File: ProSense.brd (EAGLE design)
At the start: 25.5 x 36.7 mm, 24 parts, among them U4 MIC2505 3.3

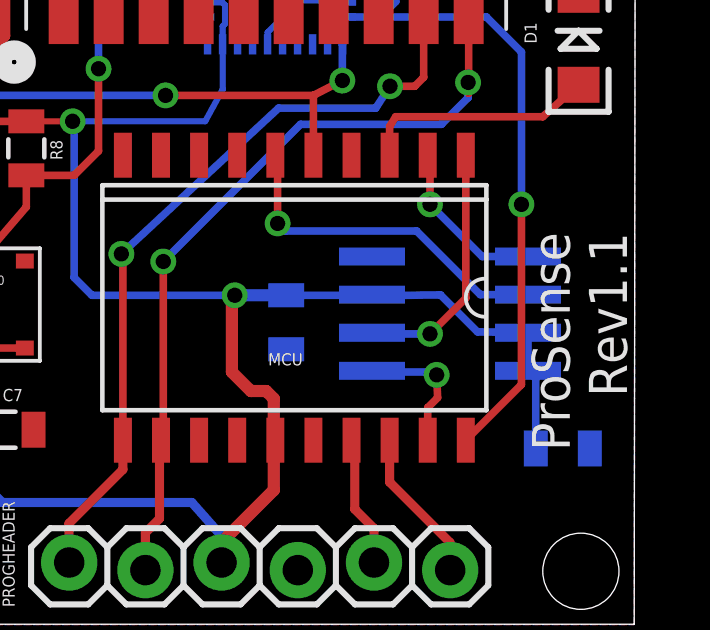
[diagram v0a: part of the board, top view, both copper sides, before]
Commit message: fixup
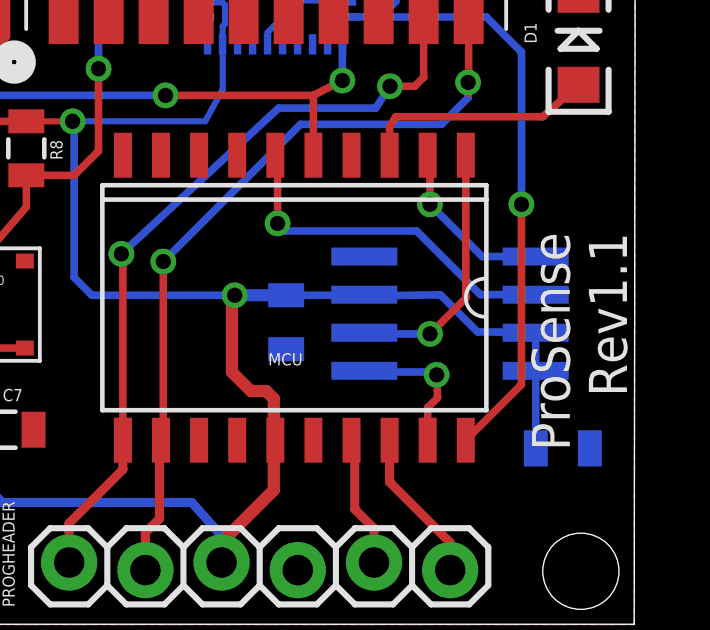
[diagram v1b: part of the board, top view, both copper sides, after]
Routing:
- net VCC: track 92.7 -> 93.3 mm
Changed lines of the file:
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@@
 <layers>
 <layer number="1" name="Top" color="4" fill="1" visible="yes" active="yes"/>
-<layer number="16" name="Bottom" color="1" fill="1" visible="yes" active="yes"/>
+<layer number="16" name="Bottom" color="1" fill="1" visible="no" active="yes"/>
 <layer number="17" name="Pads" color="2" fill="1" visible="yes" active="yes"/>
 <layer number="18" name="Vias" color="2" fill="1" visible="yes" active="yes"/>
@@
 <layer number="20" name="Dimension" color="15" fill="1" visible="yes" active="yes"/>
 <layer number="21" name="tPlace" color="16" fill="1" visible="yes" active="yes"/>
-<layer number="22" name="bPlace" color="14" fill="1" visible="yes" active="yes"/>
+<layer number="22" name="bPlace" color="14" fill="1" visible="no" active="yes"/>
 <layer number="23" name="tOrigins" color="15" fill="1" visible="yes" active="yes"/>
-<layer number="24" name="bOrigins" color="15" fill="1" visible="yes" active="yes"/>
+<layer number="24" name="bOrigins" color="15" fill="1" visible="no" active="yes"/>
 <layer number="25" name="tNames" color="7" fill="1" visible="yes" active="yes"/>
-<layer number="26" name="bNames" color="7" fill="1" visible="yes" active="yes"/>
+<layer number="26" name="bNames" color="7" fill="1" visible="no" active="yes"/>
 <layer number="27" name="tValues" color="7" fill="1" visible="no" active="yes"/>
 <layer number="28" name="bValues" color="7" fill="1" visible="no" active="yes"/>
@@
 <layer number="110" name="fp0" color="7" fill="1" visible="no" active="yes"/>
 <layer number="111" name="LPC17xx" color="7" fill="1" visible="no" active="yes"/>
-<layer number="112" name="tSilk" color="7" fill="1" visible="yes" active="yes"/>
+<layer number="112" name="tSilk" color="7" fill="1" visible="no" active="yes"/>
 <layer number="113" name="IDFDebug" color="7" fill="1" visible="no" active="yes"/>
 <layer number="114" name="FRNTMAAT1" color="7" fill="1" visible="no" active="yes"/>
@@
 <wire x1="49.18945" y1="53.23905" x2="50.408" y2="54.4576" width="0.2032" layer="16"/>
 <wire x1="49.30775" y1="40.14935" x2="52.148" y2="40.14935" width="0.254" layer="16"/>
-<wire x1="52.148" y1="40.14935" x2="52.16875" y2="40.1701" width="0.254" layer="16"/>
-<wire x1="52.16875" y1="40.1701" x2="52.20685" y2="40.132" width="0.254" layer="16"/>
+<wire x1="52.148" y1="40.14935" x2="51.91475" y2="40.1701" width="0.254" layer="16"/>
+<wire x1="51.91475" y1="40.1701" x2="52.20685" y2="40.132" width="0.254" layer="16"/>
 <wire x1="52.20685" y1="40.132" x2="54.45125" y2="40.16375" width="0.254" layer="16"/>
 <wire x1="54.45125" y1="40.16375" x2="55.68315" y2="38.93185" width="0.254" layer="16"/>
-<wire x1="55.68315" y1="38.93185" x2="57.36875" y2="38.9001" width="0.254" layer="16"/>
-<wire x1="57.36875" y1="38.9001" x2="57.36875" y2="37.6301" width="0.254" layer="16"/>
-<wire x1="57.36875" y1="37.6301" x2="57.62795" y2="37.3709" width="0.254" layer="16"/>
+<wire x1="55.68315" y1="38.93185" x2="57.62275" y2="38.9001" width="0.254" layer="16"/>
+<wire x1="57.62275" y1="38.9001" x2="57.62275" y2="37.6301" width="0.254" layer="16"/>
+<wire x1="57.62275" y1="37.6301" x2="57.62795" y2="37.3709" width="0.254" layer="16"/>
 <wire x1="57.62795" y1="37.3709" x2="57.62795" y2="35.04565" width="0.254" layer="16"/>
 <wire x1="39.09695" y1="38.3899" x2="39.08595" y2="38.30565" width="0.254" layer="1"/>
@@
 <contactref element="W25Q128FV" pad="1"/>
 <contactref element="MCU" pad="19"/>
-<wire x1="52.16875" y1="37.6301" x2="52.20685" y2="37.592" width="0.254" layer="16"/>
+<wire x1="51.91475" y1="37.6301" x2="52.20685" y2="37.592" width="0.254" layer="16"/>
 <via x="54.32425" y="37.49675" extent="1-16" drill="0.508"/>
 <wire x1="54.0258" y1="35.3185" x2="54.0258" y2="36.40455" width="0.254" layer="1"/>
@@
 <contactref element="W25Q128FV" pad="2"/>
 <contactref element="MCU" pad="1"/>
-<wire x1="52.16875" y1="38.9001" x2="52.20685" y2="38.862" width="0.254" layer="16"/>
+<wire x1="51.91475" y1="38.9001" x2="52.20685" y2="38.862" width="0.254" layer="16"/>
 <wire x1="52.20685" y1="38.862" x2="54.102" y2="38.862" width="0.254" layer="16"/>
 <via x="54.102" y="38.862" extent="1-16" drill="0.508"/>
@@
 <wire x1="49.276" y1="42.291" x2="53.6575" y2="42.291" width="0.254" layer="16"/>
 <wire x1="53.6575" y1="42.291" x2="55.7784" y2="40.1701" width="0.254" layer="16"/>
-<wire x1="55.7784" y1="40.1701" x2="57.36875" y2="40.1701" width="0.254" layer="16"/>
+<wire x1="55.7784" y1="40.1701" x2="57.62275" y2="40.1701" width="0.254" layer="16"/>
 </signal>
 <signal name="WS_DI">
@@
 <via x="54.102" y="43.18" extent="1-16" drill="0.508"/>
 <wire x1="54.102" y1="43.18" x2="55.8419" y2="41.4401" width="0.254" layer="16"/>
-<wire x1="55.8419" y1="41.4401" x2="57.36875" y2="41.4401" width="0.254" layer="16"/>
+<wire x1="55.8419" y1="41.4401" x2="57.62275" y2="41.4401" width="0.254" layer="16"/>
 </signal>
 <signal name="N$10">
